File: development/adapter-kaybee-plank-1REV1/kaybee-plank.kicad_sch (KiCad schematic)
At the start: 27 parts, among them J1 Mini-DIN-6, J2 Conn_01x10, J3 Conn_01x10, J4 Mini-DIN-6, J5 USB_A, J7 TYPE-C-31-M-12, J8 Conn_01x02_Pin, J9 Conn_01x02_Pin, Q401 BCM857BS-7-F, Q402 BC2301T 2.8A, SW1 SW_SPDT

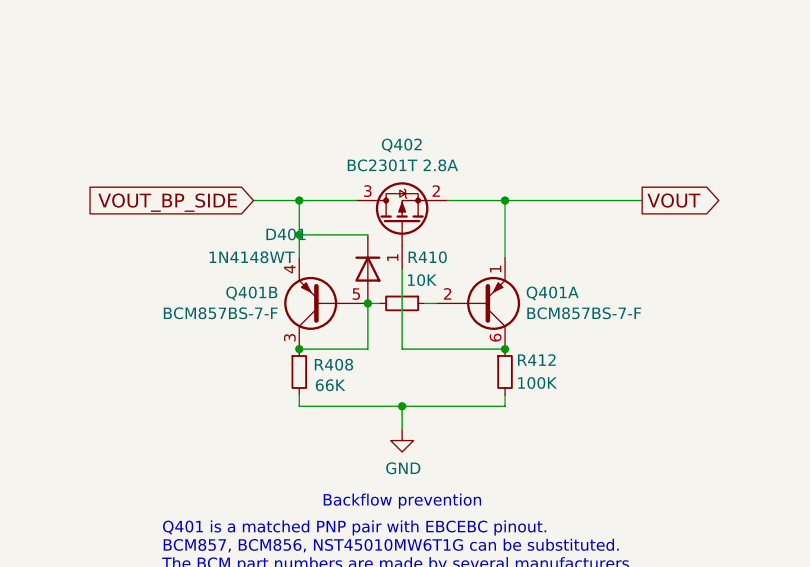
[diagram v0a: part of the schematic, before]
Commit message: kaybee production package
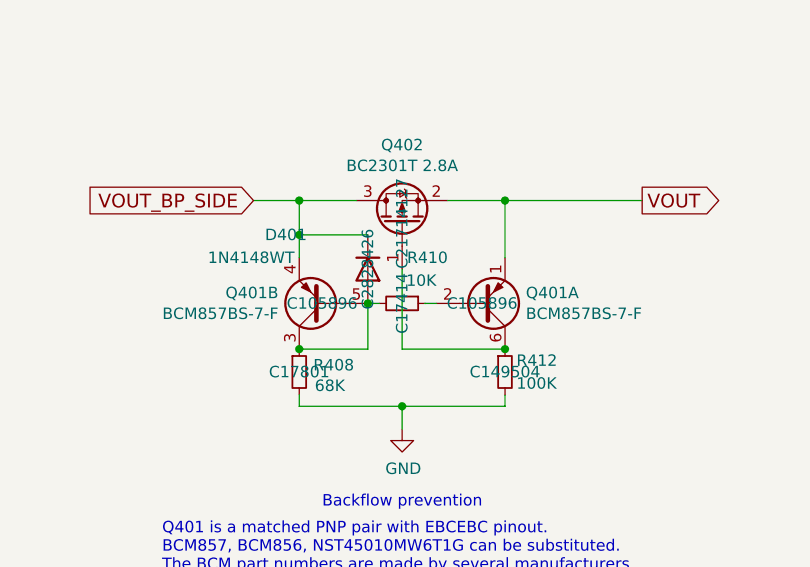
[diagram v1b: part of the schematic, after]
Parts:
- D401: szlcsc_partnum (none) -> C2828426
- Q401: szlcsc_partnum (none) -> C105896
- Q402: szlcsc_partnum (none) -> C21714127
- R408: value 66K -> 68K; szlcsc_partnum (none) -> C17801
- R410: szlcsc_partnum (none) -> C17414
- R412: szlcsc_partnum (none) -> C149504
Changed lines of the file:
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@@
+			)
+		)
+		(property "szlcsc_partnum" "C2828426"
+			(at 200.66 105.41 0)
+			(effects
+				(font
+					(size 1.27 1.27)
+				)
 			)
 		)
@@
 				)
 				(hide yes)
+			)
+		)
+		(property "szlcsc_partnum" "C17414"
+			(at 204.47 109.22 0)
+			(effects
+				(font
+					(size 1.27 1.27)
+				)
 			)
 		)
@@
 			)
 		)
-		(property "Value" "66K"
+		(property "Value" "68K"
 			(at 198.12 118.364 0)
 			(effects
@@
 				)
 				(hide yes)
+			)
+		)
+		(property "szlcsc_partnum" "C17801"
+			(at 193.04 116.84 0)
+			(effects
+				(font
+					(size 1.27 1.27)
+				)
 			)
 		)
@@
 			)
 		)
+		(property "szlcsc_partnum" "C105896"
+			(at 195.58 109.22 0)
+			(effects
+				(font
+					(size 1.27 1.27)
+				)
+			)
+		)
 		(pin "1"
 		)
@@
 			)
 		)
+		(property "szlcsc_partnum" "C105896"
+			(at 213.36 109.22 0)
+			(effects
+				(font
+					(size 1.27 1.27)
+				)
+			)
+		)
 		(pin "1"
 		)
@@
 				)
 				(hide yes)
+			)
+		)
+		(property "szlcsc_partnum" "C21714127"
+			(at 204.47 100.33 0)
+			(effects
+				(font
+					(size 1.27 1.27)
+				)
 			)
 		)
@@
 			)
 		)
+		(property "szlcsc_partnum" "C149504"
+			(at 215.9 116.84 0)
+			(effects
+				(font
+					(size 1.27 1.27)
+				)
+			)
+		)
